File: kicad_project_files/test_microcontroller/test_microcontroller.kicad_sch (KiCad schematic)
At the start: 40 parts, among them J1 USB_C_Receptacle_USB2.0, SW1 SW_Push, SW2 SW_Push, SW3 SW_Push, SW4 SW_Push, SW5 SW_Push, SW6 SW_Push, SW7 SW_Push, SW8 SW_Push, SW9 SW_Push, U1 ATmega8U2-A, Y1 16mhz

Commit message: prof_pcb
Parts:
- SW2, SW3, SW4, SW5, SW6, SW7, SW8, SW9, SW_CAPS1: footprint Button_Switch_THT:SW_PUSH_6mm -> Button - Alternate:SW_4-1437565-0
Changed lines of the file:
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@@
     (property "Reference" "SW8" (id 0) (at 72.39 80.01 0))
     (property "Value" "SW_Push" (id 1) (at 72.39 82.55 0))
-    (property "Footprint" "Button_Switch_THT:SW_PUSH_6mm" (id 2) (at 72.39 82.55 0)
+    (property "Footprint" "Button - Alternate:SW_4-1437565-0" (id 2) (at 72.39 82.55 0)
       (effects (font (size 1.27 1.27)) hide)
     )
@@
     (property "Reference" "SW_CAPS1" (id 0) (at 72.39 123.19 0))
     (property "Value" "SW_Push" (id 1) (at 72.39 125.73 0))
-    (property "Footprint" "Button_Switch_THT:SW_PUSH_6mm" (id 2) (at 72.39 125.73 0)
+    (property "Footprint" "Button - Alternate:SW_4-1437565-0" (id 2) (at 72.39 125.73 0)
       (effects (font (size 1.27 1.27)) hide)
     )
@@
     (property "Reference" "SW7" (id 0) (at 52.07 123.19 0))
     (property "Value" "SW_Push" (id 1) (at 52.07 125.73 0))
-    (property "Footprint" "Button_Switch_THT:SW_PUSH_6mm" (id 2) (at 52.07 125.73 0)
+    (property "Footprint" "Button - Alternate:SW_4-1437565-0" (id 2) (at 52.07 125.73 0)
       (effects (font (size 1.27 1.27)) hide)
     )
@@
     (property "Reference" "SW2" (id 0) (at 33.02 80.01 0))
     (property "Value" "SW_Push" (id 1) (at 33.02 82.55 0))
-    (property "Footprint" "Button_Switch_THT:SW_PUSH_6mm" (id 2) (at 33.02 82.55 0)
+    (property "Footprint" "Button - Alternate:SW_4-1437565-0" (id 2) (at 33.02 82.55 0)
       (effects (font (size 1.27 1.27)) hide)
     )
@@
     (property "Reference" "SW4" (id 0) (at 33.02 123.19 0))
     (property "Value" "SW_Push" (id 1) (at 33.02 125.73 0))
-    (property "Footprint" "Button_Switch_THT:SW_PUSH_6mm" (id 2) (at 33.02 125.73 0)
+    (property "Footprint" "Button - Alternate:SW_4-1437565-0" (id 2) (at 33.02 125.73 0)
       (effects (font (size 1.27 1.27)) hide)
     )
@@
     (property "Reference" "SW6" (id 0) (at 52.07 101.6 0))
     (property "Value" "SW_Push" (id 1) (at 52.07 104.14 0))
-    (property "Footprint" "Button_Switch_THT:SW_PUSH_6mm" (id 2) (at 52.07 104.14 0)
+    (property "Footprint" "Button - Alternate:SW_4-1437565-0" (id 2) (at 52.07 104.14 0)
       (effects (font (size 1.27 1.27)) hide)
     )
@@
     (property "Reference" "SW3" (id 0) (at 33.02 101.6 0))
     (property "Value" "SW_Push" (id 1) (at 33.02 104.14 0))
-    (property "Footprint" "Button_Switch_THT:SW_PUSH_6mm" (id 2) (at 33.02 104.14 0)
+    (property "Footprint" "Button - Alternate:SW_4-1437565-0" (id 2) (at 33.02 104.14 0)
       (effects (font (size 1.27 1.27)) hide)
     )
@@
     (property "Reference" "SW9" (id 0) (at 72.39 101.6 0))
     (property "Value" "SW_Push" (id 1) (at 72.39 104.14 0))
-    (property "Footprint" "Button_Switch_THT:SW_PUSH_6mm" (id 2) (at 72.39 104.14 0)
+    (property "Footprint" "Button - Alternate:SW_4-1437565-0" (id 2) (at 72.39 104.14 0)
       (effects (font (size 1.27 1.27)) hide)
     )
@@
     (property "Reference" "SW5" (id 0) (at 52.07 80.01 0))
     (property "Value" "SW_Push" (id 1) (at 52.07 82.55 0))
-    (property "Footprint" "Button_Switch_THT:SW_PUSH_6mm" (id 2) (at 52.07 82.55 0)
+    (property "Footprint" "Button - Alternate:SW_4-1437565-0" (id 2) (at 52.07 82.55 0)
       (effects (font (size 1.27 1.27)) hide)
     )
@@
     )
     (path "/50ca629d-9549-4245-916f-2c4cae7c3f0a"
-      (reference "SW2") (unit 1) (value "SW_Push") (footprint "Button_Switch_THT:SW_PUSH_6mm")
+      (reference "SW2") (unit 1) (value "SW_Push") (footprint "Button - Alternate:SW_4-1437565-0")
     )
     (path "/9d7818bd-ddf7-4bad-b3c0-3aef487c2b7e"
-      (reference "SW3") (unit 1) (value "SW_Push") (footprint "Button_Switch_THT:SW_PUSH_6mm")
+      (reference "SW3") (unit 1) (value "SW_Push") (footprint "Button - Alternate:SW_4-1437565-0")
     )
     (path "/52d68fde-e730-4933-938c-d2c86e1b0ff1"
-      (reference "SW4") (unit 1) (value "SW_Push") (footprint "Button_Switch_THT:SW_PUSH_6mm")
+      (reference "SW4") (unit 1) (value "SW_Push") (footprint "Button - Alternate:SW_4-1437565-0")
     )
     (path "/f6abcdb5-c97b-4658-bdd0-3f9075e03d37"
-      (reference "SW5") (unit 1) (value "SW_Push") (footprint "Button_Switch_THT:SW_PUSH_6mm")
+      (reference "SW5") (unit 1) (value "SW_Push") (footprint "Button - Alternate:SW_4-1437565-0")
     )
     (path "/94f93b90-d7fb-4cff-b857-216e3985a961"
-      (reference "SW6") (unit 1) (value "SW_Push") (footprint "Button_Switch_THT:SW_PUSH_6mm")
+      (reference "SW6") (unit 1) (value "SW_Push") (footprint "Button - Alternate:SW_4-1437565-0")
     )
     (path "/4a9040f1-6dd6-41a1-895e-666cce1f9166"
-      (reference "SW7") (unit 1) (value "SW_Push") (footprint "Button_Switch_THT:SW_PUSH_6mm")
+      (reference "SW7") (unit 1) (value "SW_Push") (footprint "Button - Alternate:SW_4-1437565-0")
     )
     (path "/03bfc24c-91fd-4454-a173-f7bf00a01ff6"
-      (reference "SW8") (unit 1) (value "SW_Push") (footprint "Button_Switch_THT:SW_PUSH_6mm")
+      (reference "SW8") (unit 1) (value "SW_Push") (footprint "Button - Alternate:SW_4-1437565-0")
     )
     (path "/c36d20a4-c7cf-4667-ac3a-a69a07598eb6"
-      (reference "SW9") (unit 1) (value "SW_Push") (footprint "Button_Switch_THT:SW_PUSH_6mm")
+      (reference "SW9") (unit 1) (value "SW_Push") (footprint "Button - Alternate:SW_4-1437565-0")
     )
     (path "/13c19b45-90cd-497a-b404-81cf9319aa9e"
-      (reference "SW_CAPS1") (unit 1) (value "SW_Push") (footprint "Button_Switch_THT:SW_PUSH_6mm")
+      (reference "SW_CAPS1") (unit 1) (value "SW_Push") (footprint "Button - Alternate:SW_4-1437565-0")
     )
     (path "/b1833f54-dfb3-49c0-a81e-48d66c89dff0"

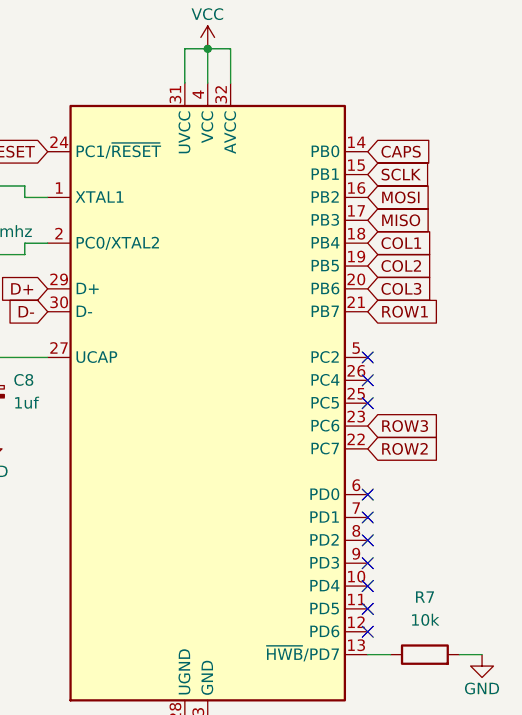
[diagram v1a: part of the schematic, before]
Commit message: pcb v1
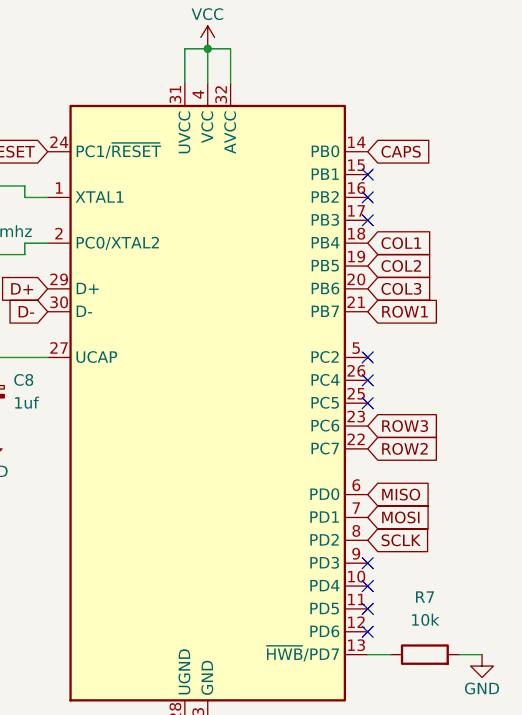
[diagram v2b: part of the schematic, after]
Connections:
- net MISO: now also U1.6 (PD0); no longer U1.17 (PB3)
- net MOSI: now also U1.7 (PD1); no longer U1.16 (PB2)
- net SCLK: now also U1.8 (PD2); no longer U1.15 (PB1)
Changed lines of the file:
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@@
   (no_connect (at 138.43 77.47))
   (no_connect (at 138.43 80.01))
+  (no_connect (at 250.19 90.17))
   (no_connect (at 250.19 107.95))
   (no_connect (at 38.1 180.34))
+  (no_connect (at 250.19 87.63))
   (no_connect (at 250.19 110.49))
-  (no_connect (at 250.19 125.73))
   (no_connect (at 250.19 130.81))
   (no_connect (at 250.19 128.27))
   (no_connect (at 250.19 133.35))
   (no_connect (at 250.19 135.89))
-  (no_connect (at 250.19 123.19))
   (no_connect (at 250.19 105.41))
-  (no_connect (at 250.19 120.65))
+  (no_connect (at 250.19 85.09))
   (wire (pts (xy 40.64 182.88) (xy 40.64 186.69))
     (stroke (width 0) (type default) (color 0 0 0 0))
@@
     )
   )
-  (global_label "SCLK" (shape input) (at 250.19 85.09 0) (fields_autoplaced)
-    (effects (font (size 1.27 1.27)) (justify left))
-    (property "Intersheet References" "${INTERSHEET_REFS}" (id 0) (at 257.3807 85.0106 0)
+  (global_label "MOSI" (shape input) (at 250.19 123.19 0) (fields_autoplaced)
+    (effects (font (size 1.27 1.27)) (justify left))
+    (property "Intersheet References" "${INTERSHEET_REFS}" (id 0) (at 257.1993 123.1106 0)
       (effects (font (size 1.27 1.27)) (justify left) hide)
     )
@@
     )
   )
+  (global_label "SCLK" (shape input) (at 250.19 125.73 0) (fields_autoplaced)
+    (effects (font (size 1.27 1.27)) (justify left))
+    (property "Intersheet References" "${INTERSHEET_REFS}" (id 0) (at 257.3807 125.6506 0)
+      (effects (font (size 1.27 1.27)) (justify left) hide)
+    )
+  )
   (global_label "ROW2" (shape input) (at 22.86 119.38 180) (fields_autoplaced)
     (effects (font (size 1.27 1.27)) (justify right))
@@
     )
   )
+  (global_label "MISO" (shape input) (at 250.19 120.65 0) (fields_autoplaced)
+    (effects (font (size 1.27 1.27)) (justify left))
+    (property "Intersheet References" "${INTERSHEET_REFS}" (id 0) (at 257.1993 120.5706 0)
+      (effects (font (size 1.27 1.27)) (justify left) hide)
+    )
+  )
   (global_label "ROW3" (shape input) (at 250.19 113.03 0) (fields_autoplaced)
     (effects (font (size 1.27 1.27)) (justify left))
@@
     )
   )
-  (global_label "MOSI" (shape input) (at 250.19 87.63 0) (fields_autoplaced)
-    (effects (font (size 1.27 1.27)) (justify left))
-    (property "Intersheet References" "${INTERSHEET_REFS}" (id 0) (at 257.1993 87.5506 0)
-      (effects (font (size 1.27 1.27)) (justify left) hide)
-    )
-  )
   (global_label "COL2" (shape input) (at 57.15 74.93 90) (fields_autoplaced)
     (effects (font (size 1.27 1.27)) (justify left))
@@
       (effects (font (size 1.27 1.27)) (justify left) hide)
     )
-  )
-  (global_label "MISO" (shape input) (at 250.19 90.17 0) (fields_autoplaced)
-    (effects (font (size 1.27 1.27)) (justify left))
-    (property "Intersheet References" "${INTERSHEET_REFS}" (id 0) (at 257.1993 90.0906 0)
-      (effects (font (size 1.27 1.27)) (justify left) hide)
-    )
